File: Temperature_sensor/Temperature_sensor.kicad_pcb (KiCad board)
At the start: 2 copper layers, 11 parts, among them IC1 TC7660, U1 TP4056, U2 ESP32-S3-ZERO

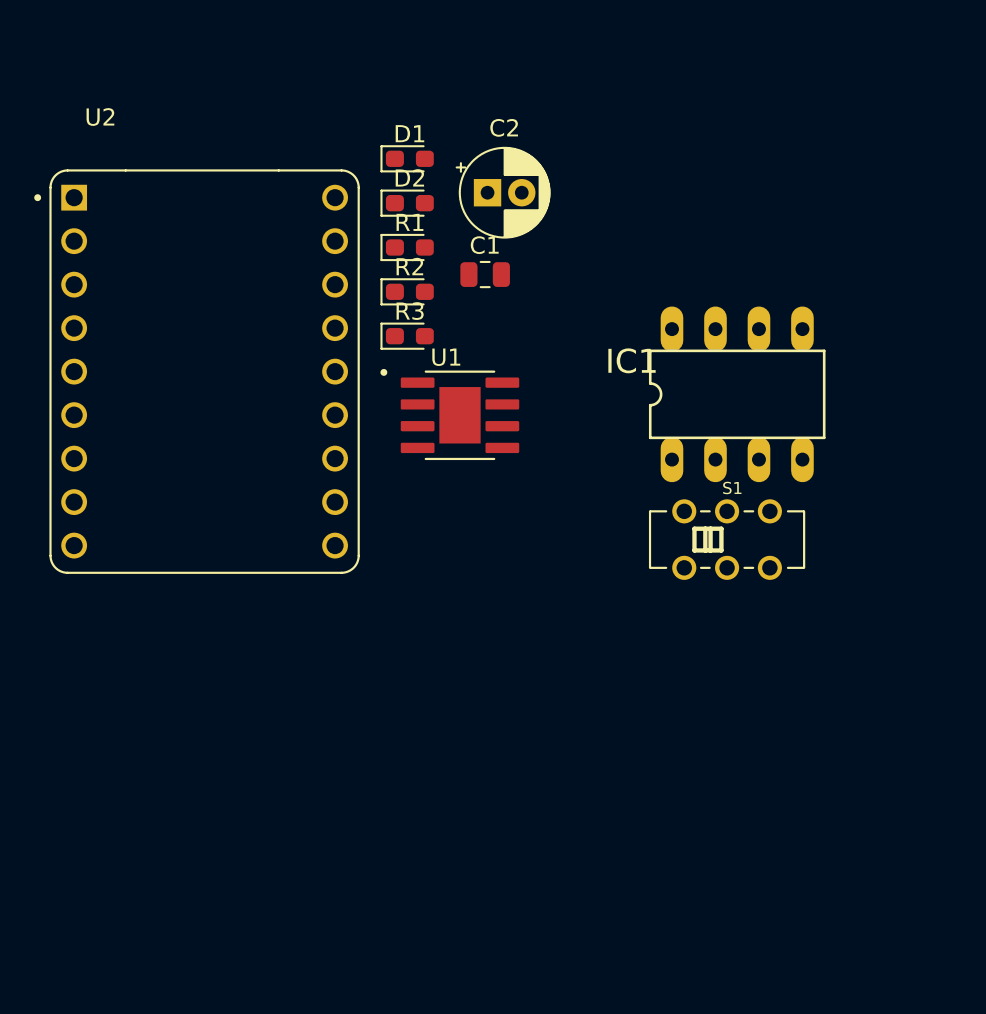
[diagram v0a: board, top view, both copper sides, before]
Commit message: final
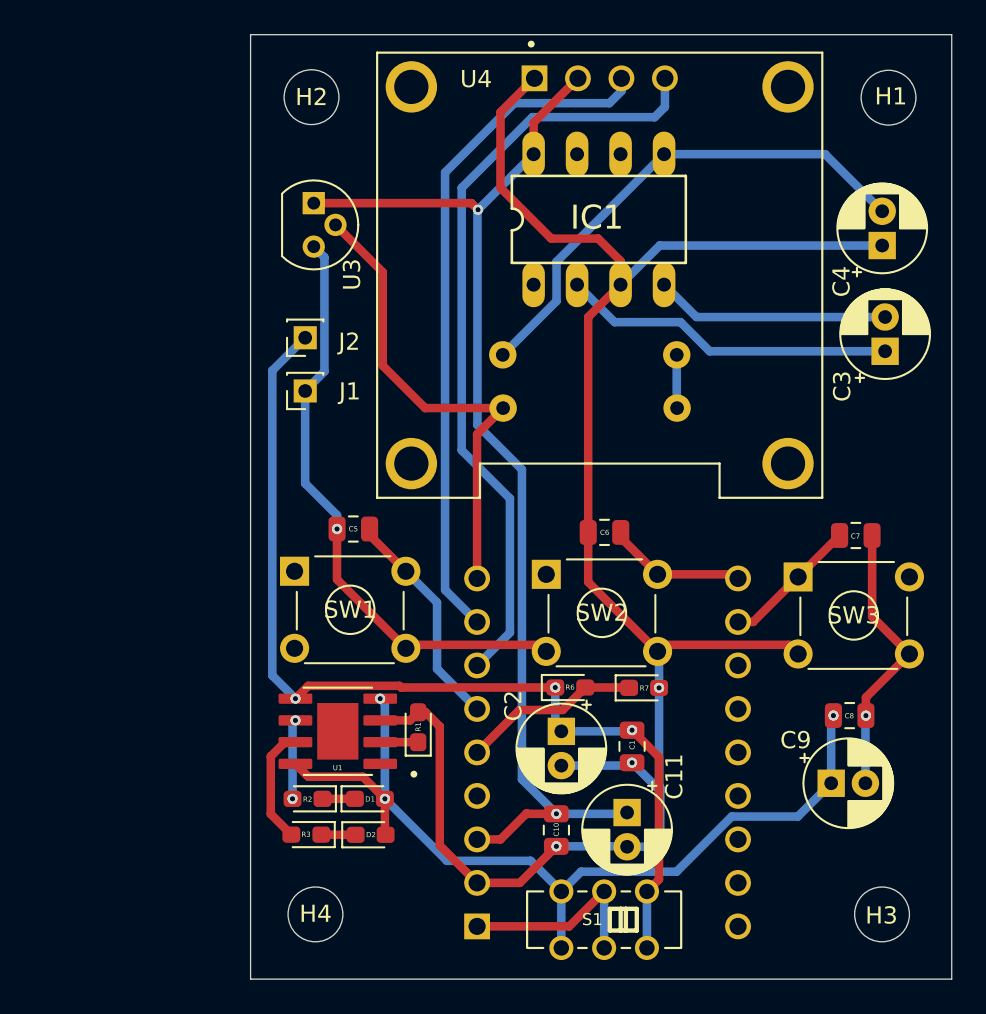
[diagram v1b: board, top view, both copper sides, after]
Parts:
- added C10: 0.1uC, Capacitor_SMD:C_0805_2012Metric, F.Cu at (137.6, 91.4)
- added C11: 22uC, Capacitor_THT:CP_Radial_D5.0mm_P2.00mm, F.Cu at (141.8, 90.4)
- added C3: 10uC, Capacitor_THT:CP_Radial_D5.0mm_P2.00mm, F.Cu at (156.8, 63.5)
- added C4: 10uC, Capacitor_THT:CP_Radial_D5.0mm_P2.00mm, F.Cu at (156.7, 57.3)
- added C5: 0.1uC, Capacitor_SMD:C_0805_2012Metric, F.Cu at (125.8, 73.8)
- added C6: 0.1uC, Capacitor_SMD:C_0805_2012Metric, F.Cu at (140.4, 74.0)
- added C7: 0.1uC, Capacitor_SMD:C_0805_2012Metric, F.Cu at (155.1, 74.2)
- added C8: 0.1uC, Capacitor_SMD:C_0805_2012Metric, F.Cu at (154.8, 84.7)
- added C9: 22uC, Capacitor_THT:CP_Radial_D5.0mm_P2.00mm, F.Cu at (153.7, 88.7)
- added H1: MountingHole, MountingHole:MountingHole_3.2mm_M3, F.Cu at (157.0, 48.6)
- added H2: MountingHole, MountingHole:MountingHole_3.2mm_M3, F.Cu at (123.3, 48.6)
- added H3: MountingHole, MountingHole:MountingHole_3.2mm_M3, F.Cu at (156.6, 96.3)
- added H4: MountingHole, MountingHole:MountingHole_3.2mm_M3, F.Cu at (123.5, 96.3)
- added J1: BAT_GND, Connector_PinSocket_2.00mm:PinSocket_1x01_P2.00mm_Vertical, F.Cu at (123.0, 65.8)
- added J2: BAT_3.7V, Connector_PinSocket_2.00mm:PinSocket_1x01_P2.00mm_Vertical, F.Cu at (123.0, 62.7)
- added R4: 47k, Resistor_THT:R_Axial_DIN0207_L6.3mm_D2.5mm_P10.16mm_Horizontal, B.Cu at (134.5, 66.8)
- added R5: 20k, Resistor_THT:R_Axial_DIN0207_L6.3mm_D2.5mm_P10.16mm_Horizontal, B.Cu at (144.7, 63.7)
- added R6: 1k, LED_SMD:LED_0603_1608Metric_Pad1.05x0.95mm_HandSolder, F.Cu at (138.4, 83.1)
- added R7: 1k, LED_SMD:LED_0603_1608Metric_Pad1.05x0.95mm_HandSolder, F.Cu at (142.7, 83.1)
- added SW1: SW_Push, SW_Push:SW_TH_Tactile_Omron_B3F-10xx, F.Cu at (122.3, 76.3)
- added SW2: SW_Push, SW_Push:SW_TH_Tactile_Omron_B3F-10xx, F.Cu at (137.0, 76.5)
- added SW3: SW_Push, SW_Push:SW_TH_Tactile_Omron_B3F-10xx, F.Cu at (151.7, 76.6)
- added U3: LM35-LP, Package_TO_SOT_THT:TO-92, F.Cu at (123.5, 54.8)
- added U4: DM-OLED096-636, OLED:MODULE_DM-OLED096-636, F.Cu at (140.2, 59.0)
- U2: moved to B.Cu
- moved D1 37.5 mm to (126.7, 89.6)
- moved D2 37.0 mm to (126.8, 91.7)
- moved U2 32.4 mm to (140.6, 86.9)
- moved C2 31.8 mm to (137.9, 85.7), turned to -90 degrees
- moved R2 30.2 mm to (123.1, 89.6), turned to 180 degrees
- moved R3 29.7 mm to (123.0, 91.7), turned to 180 degrees
- moved C1 28.9 mm to (142.0, 86.5), turned to -90 degrees
- moved R1 28.0 mm to (129.6, 85.4), turned to 90 degrees
- moved S1 23.3 mm to (140.4, 96.7), turned to 180 degrees
- moved U1 19.8 mm to (124.9, 85.6), turned to 180 degrees
- moved IC1 13.0 mm to (140.1, 55.8)
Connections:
- C1 pad 1: Net-(U1-BAT) -> BAT
- C2 pad 1: Net-(U1-BAT) -> BAT
- IC1 pad 2: unconnected-(IC1-CAP+-Pad2) -> Net-(IC1-CAP+)
- IC1 pad 3: unconnected-(IC1-GND-Pad3) -> 0
- IC1 pad 4: unconnected-(IC1-CAP--Pad4) -> Net-(IC1-CAP-)
- IC1 pad 5: unconnected-(IC1-VOUT-Pad5) -> Net-(IC1-VOUT)
- IC1 pad 8: unconnected-(IC1-V+-Pad8) -> 3.3V
- S1 pad 1: unconnected-(S1-Pad1) -> BAT
- S1 pad 2: unconnected-(S1-Pad2) -> Net-(S1-Pad2)
- S1 pad 3: unconnected-(S1-Pad3) -> 5V
- S1 pad 4: unconnected-(S1-Pad4) -> BAT
- S1 pad 5: unconnected-(S1-Pad5) -> Net-(S1-Pad2)
- S1 pad 6: unconnected-(S1-Pad6) -> 5V
- U1 pad 5: Net-(U1-BAT) -> BAT
- U2 pad 2: unconnected-(U2-GP2-Pad2) -> Chek_BAT
- U2 pad 3: unconnected-(U2-GP3-Pad3) -> GP3
- U2 pad 3V3: unconnected-(U2-3V3(OUT)-Pad3V3) -> 3.3V
- U2 pad 4: unconnected-(U2-GP4-Pad4) -> SDA
- U2 pad 5: unconnected-(U2-GP5-Pad5) -> SCL
- U2 pad 5V: 5V -> Net-(S1-Pad2)
- U2 pad 6: unconnected-(U2-GP6-Pad6) -> ADC
- U2 pad 7: unconnected-(U2-GP7-Pad7) -> GP7
- U2 pad 8: unconnected-(U2-GP8-Pad8) -> GP8
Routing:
- net 0: track 0.00 -> 180.5 mm, vias 0 -> 5
- net 3.3V: track 0.00 -> 66.6 mm, vias 0 -> 2
- net BAT: track 0.00 -> 58.5 mm, vias 0 -> 3
- net 5V: track 0.00 -> 52.4 mm, vias 0 -> 3
- net SDA: track 0.00 -> 45.4 mm
- net SCL: track 0.00 -> 40.0 mm
- net Net-(IC1-VOUT): track 0.00 -> 29.7 mm
- net ADC: track 0.00 -> 28.0 mm
- net GP3: track 0.00 -> 19.6 mm
- net Net-(IC1-CAP+): track 0.00 -> 19.6 mm
- net GP7: track 0.00 -> 14.6 mm
- net GP8: track 0.00 -> 14.5 mm
- net Net-(IC1-CAP-): track 0.00 -> 13.7 mm
- net Net-(S1-Pad2): track 0.00 -> 11.6 mm
- net Chek_BAT: track 0.00 -> 10.5 mm
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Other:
- board outline added: 41 x 55.2 mm
- copper layers 2 -> 4
